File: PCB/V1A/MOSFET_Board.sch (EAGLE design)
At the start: 267 parts, among them J201 TEMP, J202 +12V, J203 CTRL, J204 FAN_MOLEX4PIN, J205 FAN_MOLEX4PIN, J206 DUT+, J207 DUT-, Q101 BC807, Q102 BC817, Q103 BC807, Q104 BC817, Q105 BC817, Q106 BC807, Q107 BC817, Q108 BC807, Q109 SIRC10DP, Q110 SIRC10DP, Q111 BC817, Q112 BC817, Q113 SIRC10DP, Q114 SIRC10DP, Q115 BC817, Q116 BC807, Q117 BC817, Q118 BC807, Q119 IXTK102N65X2, Q120 IXTK102N65X2, Q201 BC817, Q202 BC817, Q301 BC807, Q302 BC807, Q303 BC807, Q304 BC807, Q305 BC807, Q306 BC807, Q307 BC807, Q308 BC807, Q309 BC807, Q310 BC807, Q311 BC807, Q312 BC807, Q313 BC807, Q314 BC807, U101 AD420, U102 AD420, U103 AD620, U104 AD620, U105 AD620, U106 AD620, U107 AD620, U108 AD620, U109 LTC1865L, U110 LTC1865L, U201 LP2985-3.1, U202 LP2985-3.1, U203 LP2985-3.1, U204 AD620, U205 78L05_TO-220AB-3-BR, U206 78L05_TO-220AB-3-BR, U207 LTC1865L, U208 LTC1865L, U209 MAX743, U301 HCPL-063N, U302 HCPL-063N, U303 HCPL-063N, U304 HCPL-063N, U305 HCPL-063N, U306 HCPL-063N, U307 HCPL-063N

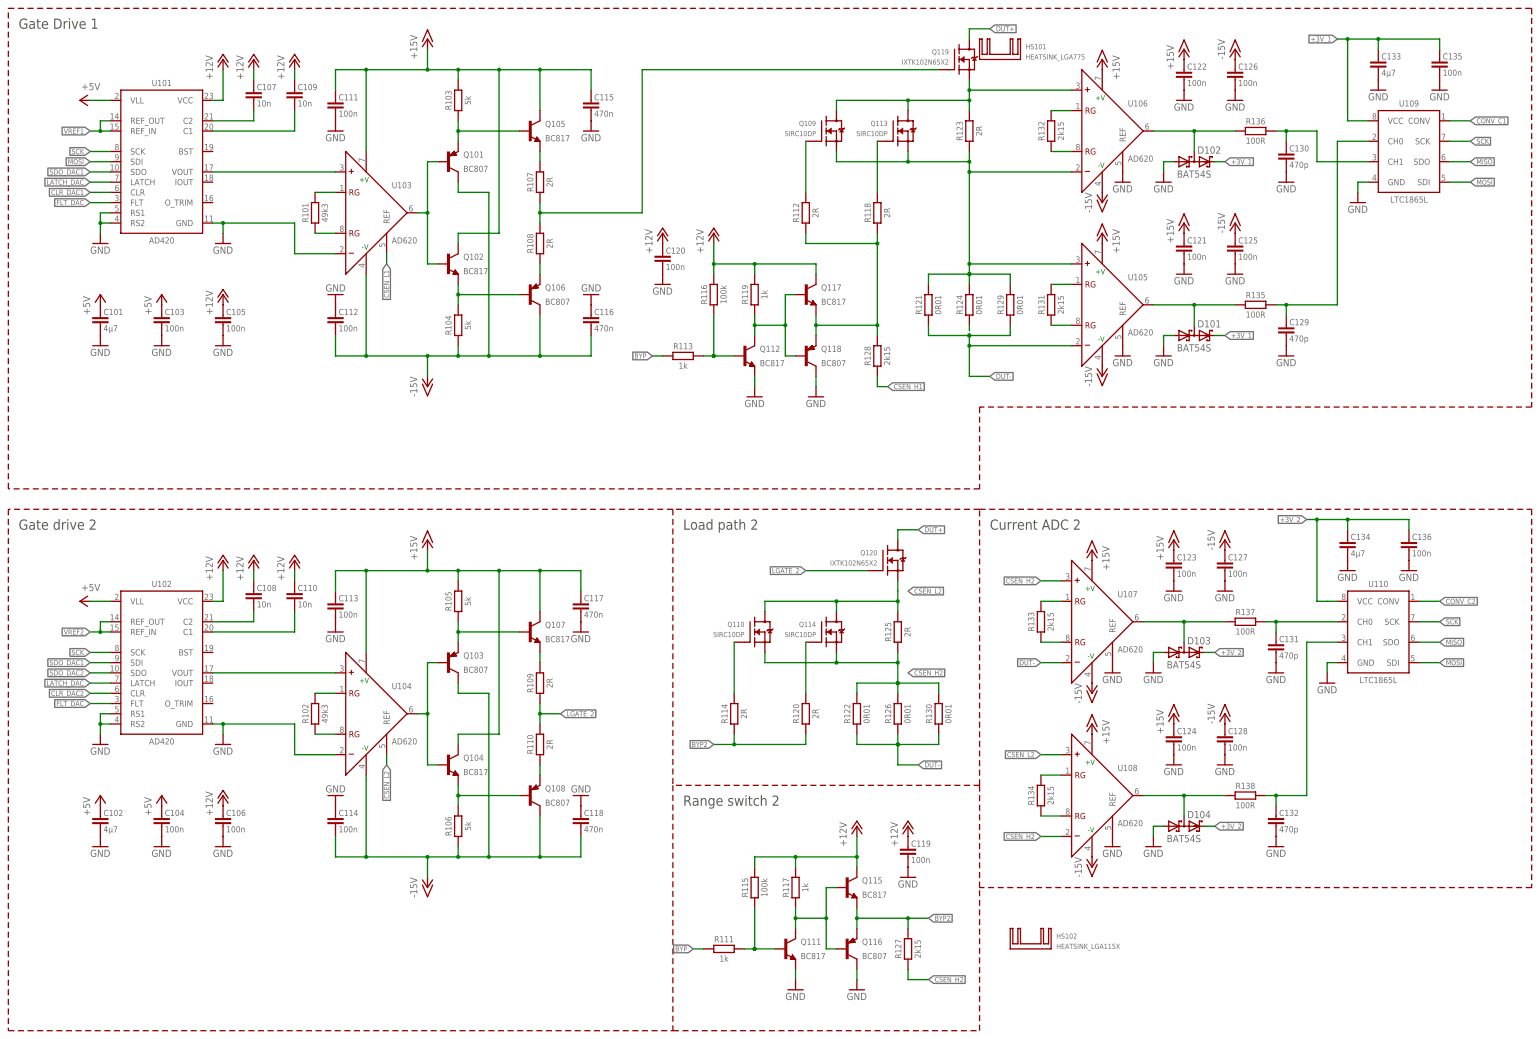
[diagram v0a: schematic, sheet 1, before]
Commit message: Schematic layout
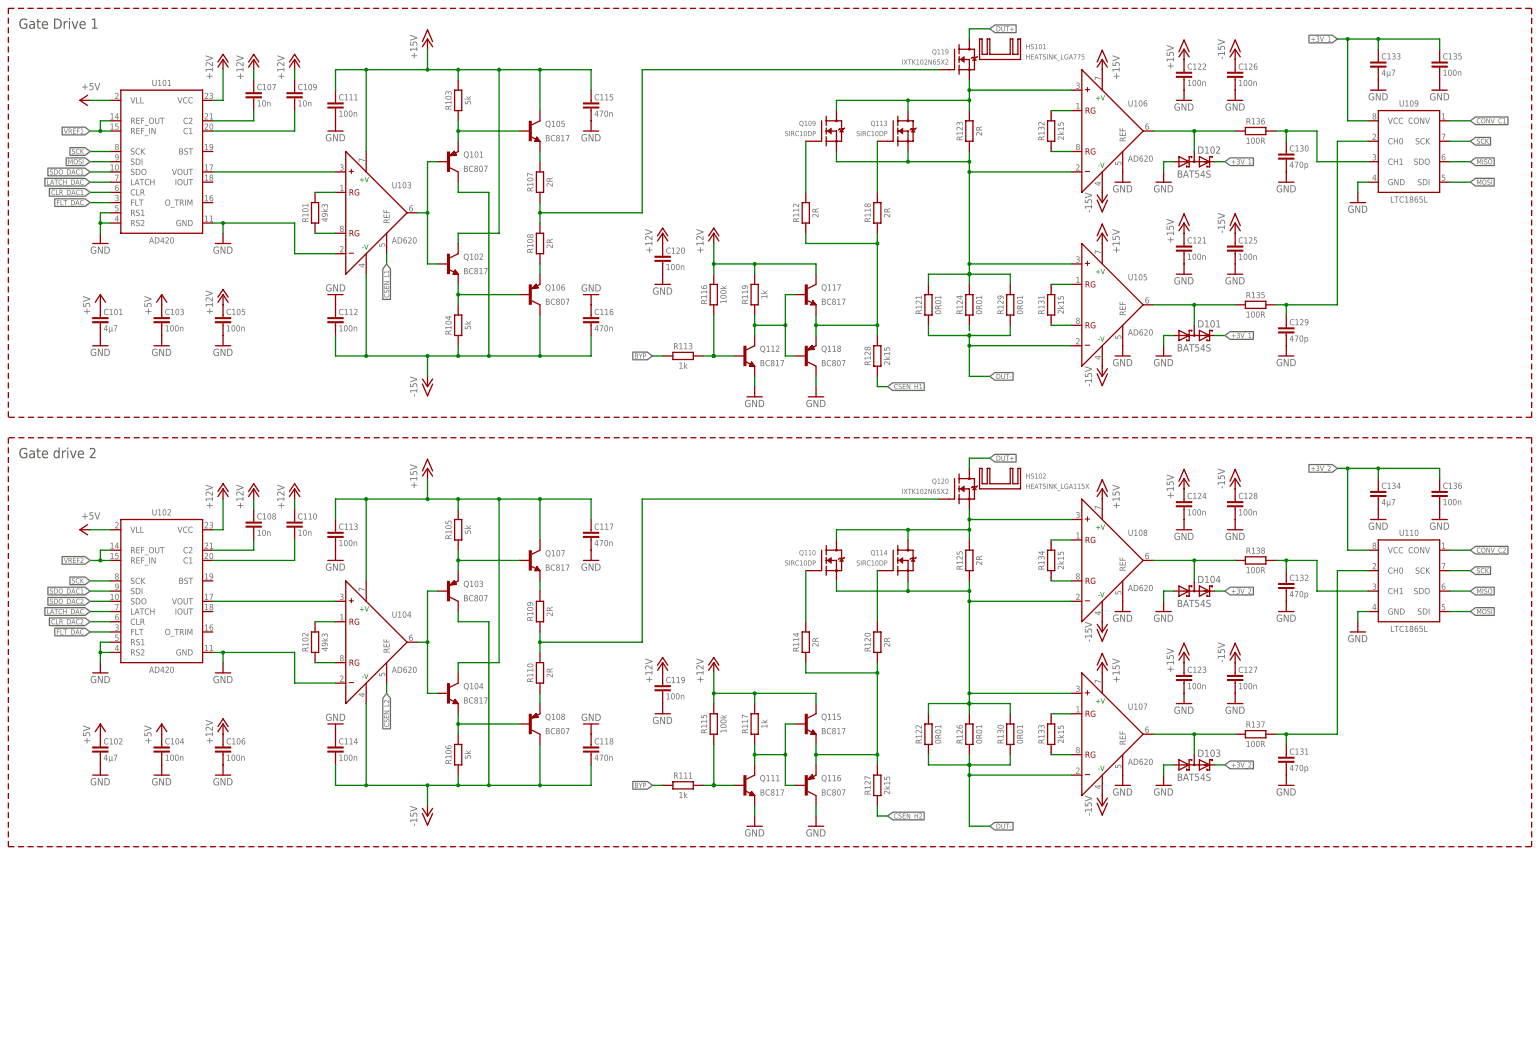
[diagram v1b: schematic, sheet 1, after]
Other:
- note removed: "Current ADC 2"
- note removed: "Load path 2"
- note removed: "Range switch 2"
- moved on the sheet: C102, C104, C106, C108, C110, C113, C114, C117, C118, C119, C123, C124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
